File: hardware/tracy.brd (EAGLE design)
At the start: 100 x 80 mm, 67 parts, among them IC1 SIM900, J1 U.FL, J2 U.FL, Q4 si2305cd, T2 BC846, U1 SPX5205 3v3, U3 TC1014 2V8, Y1 32768Hz CFPX-217 12.5pF

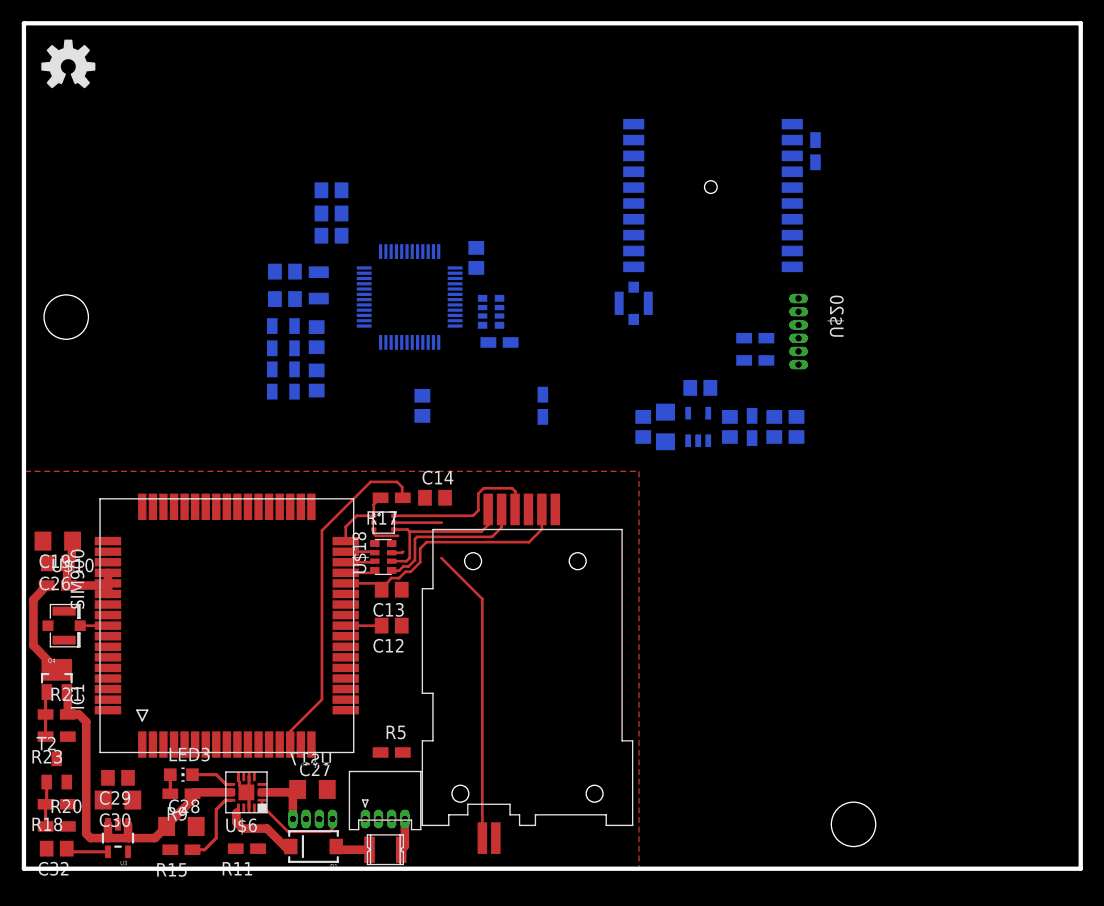
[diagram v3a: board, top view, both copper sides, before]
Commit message: pcb done
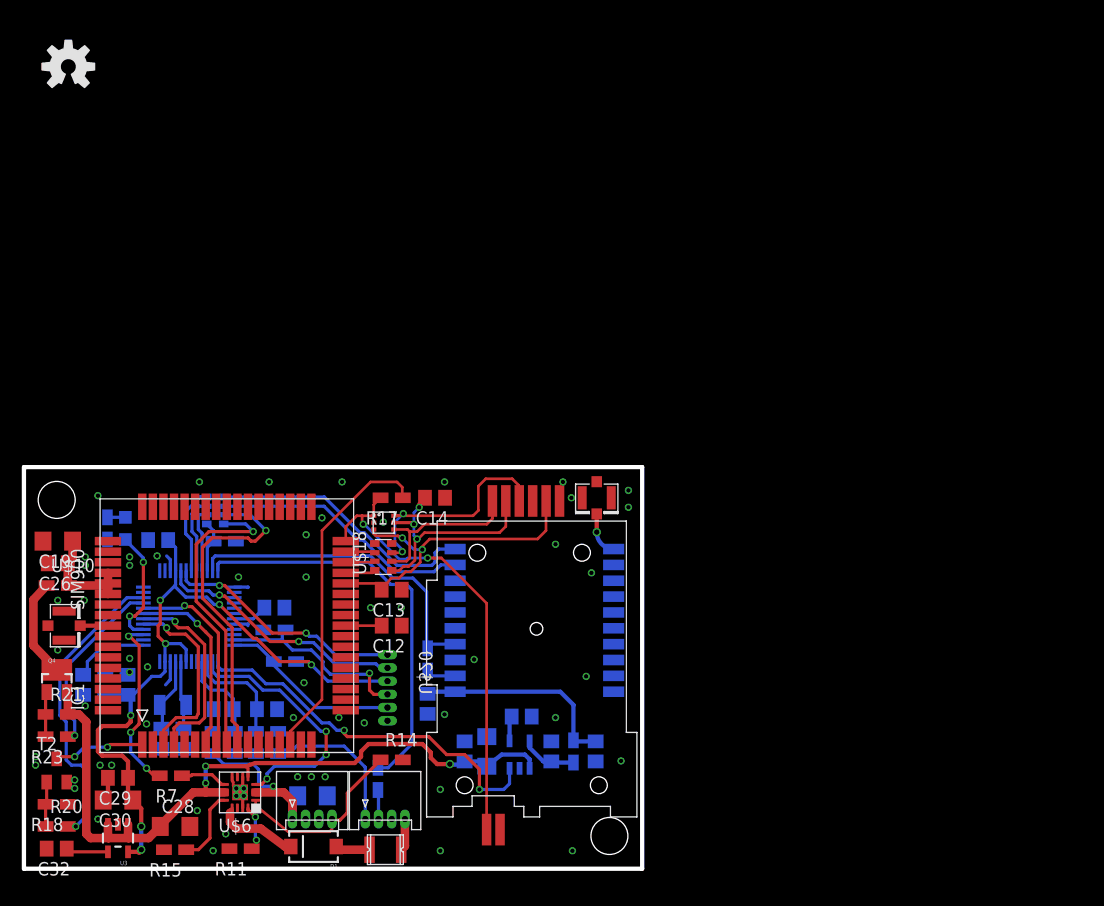
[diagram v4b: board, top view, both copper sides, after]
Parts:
- removed LED3: orange, led:CHIP-LED0805
- removed R9: 10k, rcl:R0805W
- added LED1: green, led:CHIPLED_0805
- added R6: 100k, rcl:R0805W
- added R7: 470, rcl:R0805W
- R14: value NA/10k -> DNP 10k th
- U$17: value battery -> MOLEX_4HORIZONTAL
- U$19: value power_in -> MOLEX_4HORIZONTAL
- U2: value (none) -> 3339
- moved R1 60.5 mm to (38.2, 19.8), turned to 90 degrees
- moved R35 53.2 mm to (23.7, 22.6), turned to 0 degrees
- moved R34 52.8 mm to (24.7, 19.6)
- moved C10 52.4 mm to (5.60, 17.4), turned to 270 degrees
- moved U$20 51.5 mm to (34.4, 14.0)
- moved C17 49.5 mm to (7.70, 17.4), turned to 270 degrees
- moved C8 46.7 mm to (9.80, 17.4), turned to 270 degrees
- moved C24 45.7 mm to (13.0, 12.3), turned to 270 degrees
- moved C7 43.6 mm to (38.2, 15.6), turned to 270 degrees
- moved C23 42.7 mm to (15.1, 12.3), turned to 270 degrees
- moved Y1 42.0 mm to (14.1, 15.5), turned to 180 degrees
- moved U2 40.8 mm to (40.3, 31.5), turned to 180 degrees
- moved C9 40.2 mm to (12.7, 31.1), turned to 180 degrees
- moved R3 39.7 mm to (18.9, 10.9), turned to 180 degrees
- moved R4 37.9 mm to (18.9, 13.0), turned to 0 degrees
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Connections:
- net N$8 renamed GPS_VCC
- removed net N$21: LED3.C, U$6.9
- removed net N$22: LED3.A, R9.2
- removed net P1.0: U$1.14
- removed net P1.1: U$1.15
- removed net P1.2: U$1.16
- removed net P1.3: U$1.17
- removed net P1.4: U$1.18
- removed net P1.5: U$1.19
- removed net P1.6: U$1.20
- removed net P1.7: U$1.21
- removed net P2.0: U$1.22
- removed net P4.6: U$1.35
- removed net P4.7: U$1.36
- removed net P5.0: U$1.5
- removed net P5.1: U$1.6
- removed net P6.0: U$1.1
- removed net P6.1: C18.1, R22.2, R24.1, U$1.2
- removed net P6.2: C2.1, R3.2, R4.1, U$1.3
- removed net P6.3: U$1.4
- new net BAT_DIV: C2.1, R3.2, R4.1, U$1.4
- new net CH: R7.2, U$1.15
- new net N$10: R7.1, U$6.9
- new net N$8: LED1.C, R6.1
- new net PW_RAW_DIV: C18.1, R22.2, R24.1, U$1.3
- new net STATUS: LED1.A, U$1.16
- net 3V3_EN: now also U$1.1
- net 5V: now also U$17.4; no longer U$19.4
- net BAT: now also U$19.1; no longer U$17.4
- net CE: now also U$1.2
- net CTS: now also U$1.19
- net DTR: now also U$1.17
- net GND: now also R6.2, U$19.2; no longer U$17.2
- net GPRS_EN: now also U$1.21
- net GPRS_POW: now also U$1.22
- net N$12: now also U$17.2; no longer U$19.2
- net P4.0: now also U$20.5; no longer U$20.6
- net P4.1: now also U$20.6; no longer U$20.5
- net PW_EN: now also U$1.36
- net PW_RAW: now also U$17.1; no longer U$19.1
- net RI: now also U$1.18
- net RTS: now also U$1.20
- net TS: now also U$19.4; no longer U$17.1
- net VBACKUP: now also U$1.35
- net VIN: no longer R9.1
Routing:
- net 2V8: track 0.00 -> 70.7 mm, vias 0 -> 7
- net PW_EN: track 0.00 -> 38.9 mm
- net VIN: track 33.4 -> 70.6 mm, vias 0 -> 3
- net 3V3_EN: track 0.00 -> 36.2 mm, vias 0 -> 2
- net GPRS_RX: track 0.00 -> 31.5 mm, vias 0 -> 1
- net VBACKUP: track 0.00 -> 30.9 mm
- net GPRS_TX: track 0.00 -> 29.2 mm, vias 0 -> 1
- net GPRS_POW: track 0.00 -> 28.6 mm, vias 0 -> 1
- net GPS_RX: track 0.00 -> 25.8 mm
- net GPS_TX: track 0.00 -> 24.7 mm
- net CE: track 0.00 -> 24.4 mm, vias 0 -> 3
- net P4.0: track 0.00 -> 24.1 mm, vias 0 -> 2
- net P4.1: track 0.00 -> 22.9 mm, vias 0 -> 2
- net GPS_VCC: track 0.00 -> 20.4 mm
- net TEST: track 0.00 -> 19.0 mm, vias 0 -> 1
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- added copper zone on layer 16, net GND
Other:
- board size 100 x 80 mm -> 58.5 x 38 mm
